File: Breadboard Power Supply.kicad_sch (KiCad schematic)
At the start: 32 parts, among them J1 USB-C Power Only, J10 Conn_01x02_Male, J11 Conn_01x02_Male, J2 Conn_01x02_Male, J3 Conn_01x02_Male, J4 Conn_01x02_Male, J5 Conn_01x02_Male, J6 Conn_01x02_Male, J7 Conn_01x02_Male, J8 Conn_01x02_Male, J9 Conn_01x02_Male, U1 LM1117-ADJ, U2 LM1117-ADJ

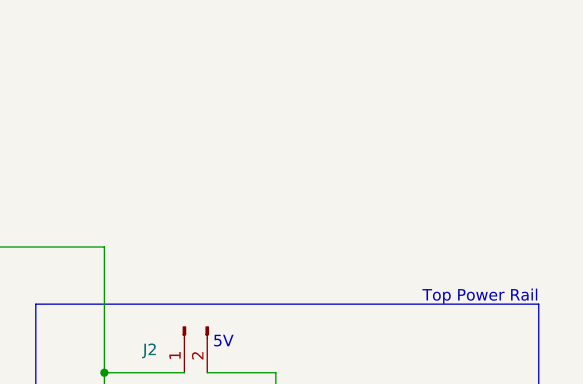
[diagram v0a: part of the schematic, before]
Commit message: Updates.
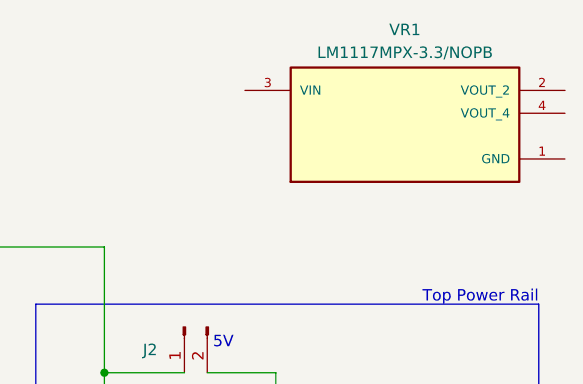
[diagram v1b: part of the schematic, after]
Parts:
- added VR1: LM1117MPX-3.3/NOPB, VREG_LM1117MPX-3.3/NOPB, symbol LM1117MPX-3.3_NOPB:LM1117MPX-3.3/NOPB
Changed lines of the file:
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@@
+    )
+  )
+  (symbol (lib_id "LM1117MPX-3.3_NOPB:LM1117MPX-3.3{slash}NOPB") (at 204.851 29.591 0) (unit 1)
+    (in_bom yes) (on_board yes) (dnp no) (fields_autoplaced)
+    (property "Reference" "VR1" (at 204.851 20.32 0)
+      (effects (font (size 1.27 1.27)))
+    )
+    (property "Value" "LM1117MPX-3.3/NOPB" (at 204.851 22.86 0)
+      (effects (font (size 1.27 1.27)))
+    )
+    (property "Footprint" "VREG_LM1117MPX-3.3/NOPB" (at 204.851 29.591 0)
+      (effects (font (size 1.27 1.27)) (justify bottom) hide)
+    )
+    (property "Datasheet" "" (at 204.851 29.591 0)
+      (effects (font (size 1.27 1.27)) hide)
+    )
+    (property "MAXIMUM_PACKAGE_HEIGHT" "1.80 mm" (at 204.851 29.591 0)
+      (effects (font (size 1.27 1.27)) (justify bottom) hide)
+    )
+    (property "STANDARD" "Manufacturer Recommendation" (at 204.851 29.591 0)
+      (effects (font (size 1.27 1.27)) (justify bottom) hide)
+    )
+    (property "PARTREV" "O" (at 204.851 29.591 0)
+      (effects (font (size 1.27 1.27)) (justify bottom) hide)
+    )
+    (property "MANUFACTURER" "Texas Instruments" (at 204.851 29.591 0)
+      (effects (font (size 1.27 1.27)) (justify bottom) hide)
+    )
+    (pin "1")
+    (pin "2")
+    (pin "3")
+    (pin "4")
+    (instances
+      (project "Breadboard Power Supply"
+        (path "/a474ae98-d5ea-4288-b242-cd0417157b2d"
+          (reference "VR1") (unit 1)
+        )
+      )
     )
   )
